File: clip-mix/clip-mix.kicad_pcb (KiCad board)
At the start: 2 copper layers, 22 parts, among them J1 Conn_01x01_Female, J2 Conn_01x01_Female, J3 Conn_01x01_Female, J4 Conn_02x05_Odd_Even, U1 TL074

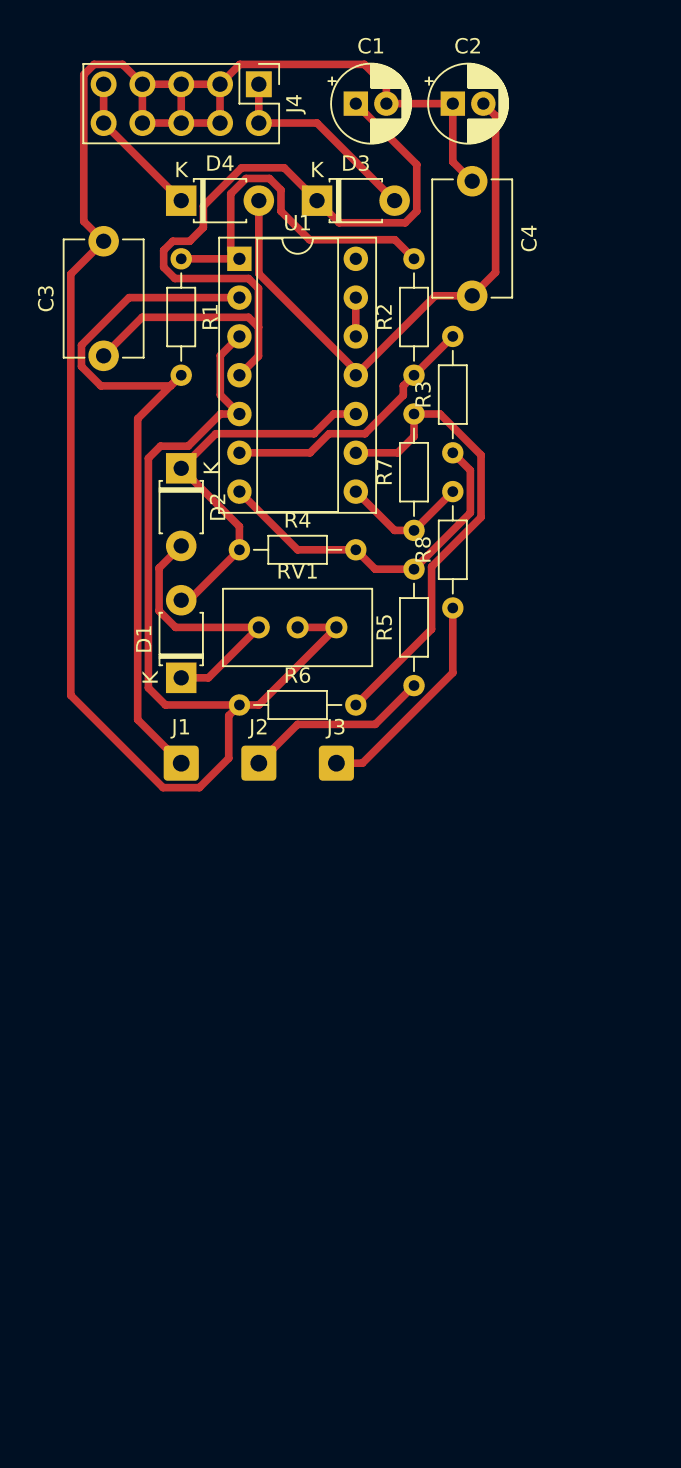
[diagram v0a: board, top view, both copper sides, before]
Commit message: work on test and clip mix
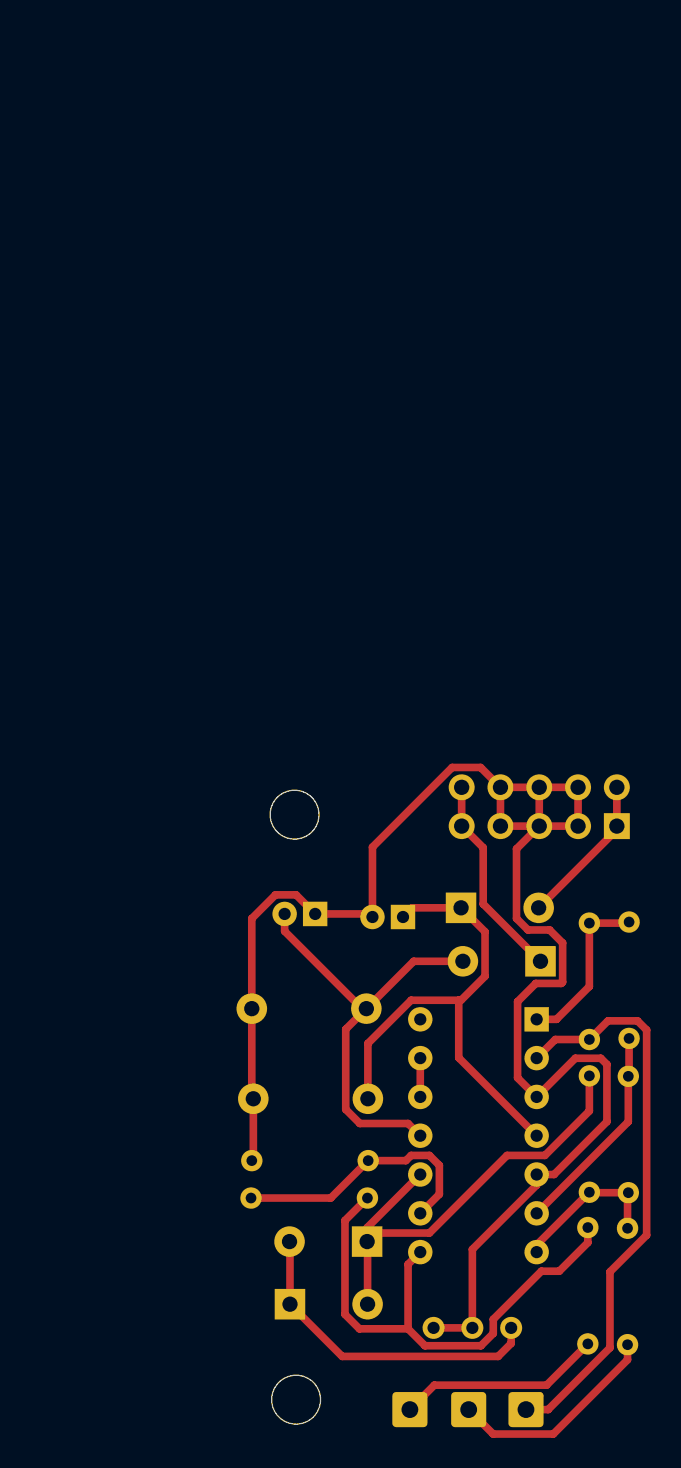
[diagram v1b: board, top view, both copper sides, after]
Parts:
- added REF**: MountingHole_3.2mm_M3, MountingHole:MountingHole_3.2mm_M3, B.Cu at (152.2, 97.3)
- added REF**: MountingHole_3.2mm_M3, MountingHole:MountingHole_3.2mm_M3, B.Cu at (152.3, 135.7)
- C1, C2: value CP1 -> 10uF; moved to B.Cu
- C3, C4: value C -> 0.1uF; moved to B.Cu
- D1, D2: value D -> 1N4148; moved to B.Cu
- D3: value D_Schottky -> 1N5189; moved to B.Cu
- D4: value D_Schottky -> 1N1589; moved to B.Cu
- J1: value Conn_01x01_Female -> IN; moved to B.Cu
- J2: value Conn_01x01_Female -> OUT; moved to B.Cu
- J3: value Conn_01x01_Female -> CLIP OUT; moved to B.Cu
- J4: value Conn_02x05_Odd_Even -> Power; moved to B.Cu
- R1, R2, R3, R4, R7: value R -> 100K; moved to B.Cu
- R5, R8: value R -> 1K; moved to B.Cu
- R6: value R -> 27K; moved to B.Cu
- RV1: value R_POT -> 20K; moved to B.Cu
- U1: moved to B.Cu
- moved C4 56.1 mm to (149.4, 110.0), turned to 0 degrees
- moved D4 55.1 mm to (168.3, 107.0), turned to 180 degrees
- moved J4 53.9 mm to (173.3, 98.1), turned to 90 degrees
- moved C2 53.8 mm to (153.6, 103.8), turned to 180 degrees
- moved U1 53.5 mm to (168.1, 110.8), turned to 180 degrees
- moved C1 53.3 mm to (159.3, 104.0), turned to 180 degrees
- moved D2 52.1 mm to (156.9, 125.3), turned to 180 degrees
- moved C3 51.6 mm to (157.0, 116.0), turned to 180 degrees
- moved R1 51.0 mm to (171.5, 104.5)
- moved R3 49.8 mm to (174.1, 122.1)
- moved R8 49.0 mm to (171.4, 132.0)
- moved J1 48.0 mm to (167.3, 136.3), turned to 180 degrees
- moved D3 47.3 mm to (163.1, 103.5)
- moved RV1 46.3 mm to (161.3, 130.9), turned to 180 degrees
- moved R2 45.6 mm to (174.1, 112.0)
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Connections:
- net Net-(D3-Pad2) renamed +12v
- net Net-(D4-Pad1) renamed -12V
- U1 pad 12: (no net) -> Net-(U1-Pad12)
- U1 pad 13: (no net) -> Net-(U1-Pad12)
- U1 pad 14: (no net) -> Net-(U1-Pad14)
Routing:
- net Earth: track 151.2 -> 111.6 mm
- net Net-(R7-Pad1): track 8.45 -> 34.7 mm
- net Net-(C1-Pad1): track 55.7 -> 33.3 mm
- net Net-(R6-Pad2): track 31.0 -> 17.5 mm
- net Net-(R3-Pad1): track 23.2 -> 10.5 mm
- net Net-(R1-Pad1): track 23.7 -> 11.1 mm
- net Net-(J1-Pad1): track 48.1 -> 39.0 mm
- net Net-(C2-Pad2): track 37.4 -> 28.9 mm
- net Net-(D1-Pad2): track 25.0 -> 30.5 mm
- net -12V: track 9.72 -> 13.5 mm
- net Net-(R2-Pad1): track 17.5 -> 14.0 mm
- net +12v: track 13.5 -> 10.0 mm
- net Net-(D1-Pad1): track 18.3 -> 21.4 mm
- net (no net): track 2.54 -> 0.00 mm
- net Net-(U1-Pad12): track 0.00 -> 2.54 mm
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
